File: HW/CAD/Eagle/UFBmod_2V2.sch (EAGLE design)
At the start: 212 parts, among them J1411 ABRACON_ARJE-0034, T0551 MMBT2222, U0501 MIDAS_MCCOG21605B6W-FPTLWI, U0601 MAX5217, U0651 LM4120IM5-3.0, U0701 AT86RF215-ZU, U0711 ASVTX-13-D-26.000MHZ-I05-T, U0811 PE4259, U0821 RFX1010, U0881 B39871B3440U410, U0911 FT232HL, U1101 TPS53353, U1211 TPS62745DSSR, X0891 ANTENNATINY, X0895 ANTENNATINY, X1011 TTE_EN11-HSM, X1311 MOLEX 105017-0001, X1351 PHOENIX_1990067_1X8X2MM50_PTS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, X1361 PHOENIX_1990067_1X8X2MM50_PTS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

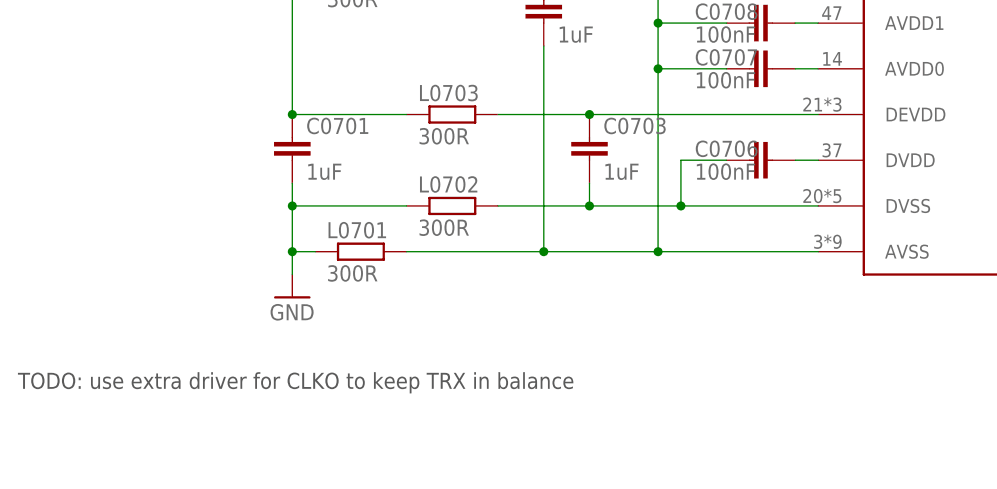
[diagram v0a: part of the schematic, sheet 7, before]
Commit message: HW - Eagle - V2.1 V2.2 - TRX no 300R inductors at GND lines
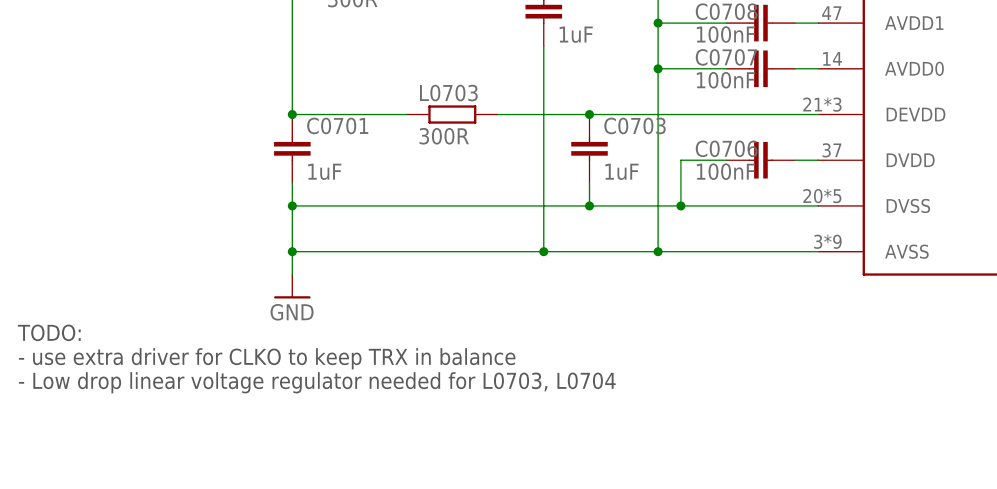
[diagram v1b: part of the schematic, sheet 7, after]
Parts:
- removed L0701, L0702: 300R, df4iah_rcl:R-EU_R1206
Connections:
- removed net TRX_AVSS: C0704.2, C0707.1, C0708.1, L0701.2, U0701.AVSS, U0701.XTAL2
- removed net TRX_DVSS: C0703.2, C0706.1, L0702.2, U0701.DVSS
- net GND: now also C0703.2, C0704.2, C0706.1, C0707.1, C0708.1, U0701.AVSS, U0701.DVSS, U0701.XTAL2; no longer L0701.1, L0702.1
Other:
- note added: "TODO: - use extra driver for CLKO to keep TRX in balance - Low drop linear voltage regulator needed for L0703, L0704"
- note removed: "TODO: use extra driver for CLKO to keep TRX in balance"
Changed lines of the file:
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@@
 <part name="FRAME_07" library="df4iah_frame" deviceset="A4L-LOC" device="" value="Holes"/>
 <part name="U0701" library="df4iah_rf" deviceset="AT86RF215" device="" value="AT86RF215-ZU"/>
-<part name="L0702" library="df4iah_rcl" deviceset="R-EU_" device="R1206" value="300R"/>
-<part name="L0701" library="df4iah_rcl" deviceset="R-EU_" device="R1206" value="300R"/>
 <part name="GND0701" library="df4iah_supply" deviceset="GND" device=""/>
 <part name="L0703" library="df4iah_rcl" deviceset="R-EU_" device="R1206" value="300R"/>
@@
 <text x="22.86" y="162.56" size="2.54" layer="97" ratio="15">Microchip Technologies AT86RF215</text>
 <text x="93.98" y="83.82" size="1.778" layer="97">26MHz</text>
-<text x="15.24" y="22.86" size="1.778" layer="97">TODO: use extra driver for CLKO to keep TRX in balance</text>
+<text x="15.24" y="22.86" size="1.778" layer="97">TODO:
+- use extra driver for CLKO to keep TRX in balance
+- Low drop linear voltage regulator needed for L0703, L0704</text>
 </plain>
 <instances>
@@
 <attribute name="VALUE" x="142.24" y="76.2" size="1.9304" layer="96" font="vector" ratio="10" rot="R90"/>
 </instance>
-<instance part="L0702" gate="G$1" x="63.5" y="43.18"/>
-<instance part="L0701" gate="G$1" x="53.34" y="38.1"/>
 <instance part="GND0701" gate="1" x="45.72" y="33.02"/>
 <instance part="L0703" gate="G$1" x="63.5" y="53.34"/>
@@
 </busses>
 <nets>
-<net name="TRX_DVSS" class="0">
-<segment>
-<pinref part="L0702" gate="G$1" pin="2"/>
+<net name="GND" class="0">
+<segment>
+<wire x1="45.72" y1="38.1" x2="45.72" y2="35.56" width="0.1524" layer="91"/>
+<wire x1="45.72" y1="38.1" x2="45.72" y2="43.18" width="0.1524" layer="91"/>
+<junction x="45.72" y="38.1"/>
+<wire x1="45.72" y1="43.18" x2="78.74" y2="43.18" width="0.1524" layer="91"/>
+<pinref part="GND0701" gate="1" pin="GND"/>
+<pinref part="C0701" gate="G$1" pin="2"/>
+<wire x1="45.72" y1="43.18" x2="45.72" y2="45.72" width="0.1524" layer="91"/>
+<junction x="45.72" y="43.18"/>
 <pinref part="U0701" gate="G$1" pin="DVSS"/>
-<wire x1="68.58" y1="43.18" x2="78.74" y2="43.18" width="0.1524" layer="91"/>
 <pinref part="C0703" gate="G$1" pin="2"/>
 <wire x1="78.74" y1="43.18" x2="88.9" y2="43.18" width="0.1524" layer="91"/>
@@
 <pinref part="C0706" gate="G$1" pin="1"/>
 <wire x1="88.9" y1="48.26" x2="93.98" y2="48.26" width="0.1524" layer="91"/>
-</segment>
-</net>
-<net name="TRX_AVSS" class="0">
-<segment>
-<pinref part="L0701" gate="G$1" pin="2"/>
 <pinref part="U0701" gate="G$1" pin="AVSS"/>
-<wire x1="58.42" y1="38.1" x2="73.66" y2="38.1" width="0.1524" layer="91"/>
+<wire x1="45.72" y1="38.1" x2="73.66" y2="38.1" width="0.1524" layer="91"/>
 <pinref part="C0704" gate="G$1" pin="2"/>
 <wire x1="73.66" y1="38.1" x2="86.36" y2="38.1" width="0.1524" layer="91"/>
@@
 <wire x1="96.52" y1="91.44" x2="104.14" y2="91.44" width="0.1524" layer="91"/>
 </segment>
-</net>
-<net name="GND" class="0">
-<segment>
-<pinref part="L0701" gate="G$1" pin="1"/>
-<wire x1="48.26" y1="38.1" x2="45.72" y2="38.1" width="0.1524" layer="91"/>
-<wire x1="45.72" y1="38.1" x2="45.72" y2="35.56" width="0.1524" layer="91"/>
-<wire x1="45.72" y1="38.1" x2="45.72" y2="43.18" width="0.1524" layer="91"/>
-<junction x="45.72" y="38.1"/>
-<pinref part="L0702" gate="G$1" pin="1"/>
-<wire x1="45.72" y1="43.18" x2="58.42" y2="43.18" width="0.1524" layer="91"/>
-<pinref part="GND0701" gate="1" pin="GND"/>
-<pinref part="C0701" gate="G$1" pin="2"/>
-<wire x1="45.72" y1="43.18" x2="45.72" y2="45.72" width="0.1524" layer="91"/>
-<junction x="45.72" y="43.18"/>
-</segment>
-<segment>
+<segment>
